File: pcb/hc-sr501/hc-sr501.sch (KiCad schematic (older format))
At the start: 35 parts, among them J1 Conector 3 pines, U1 BISS0001, U2 HT7133-1

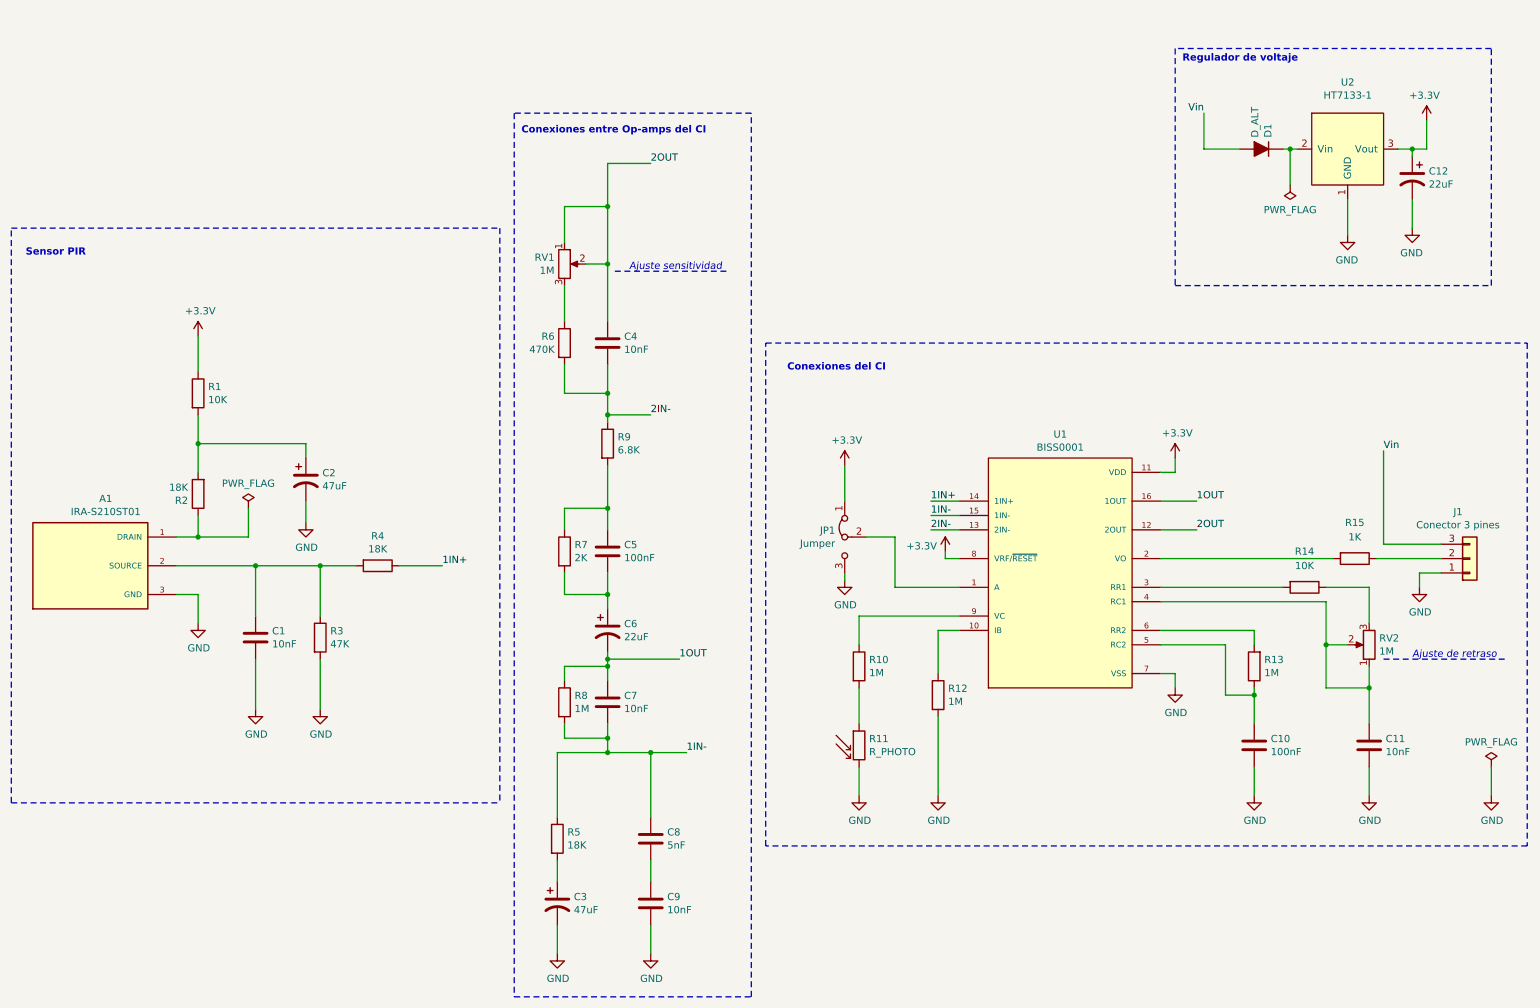
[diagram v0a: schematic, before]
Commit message: Cambios de PCB
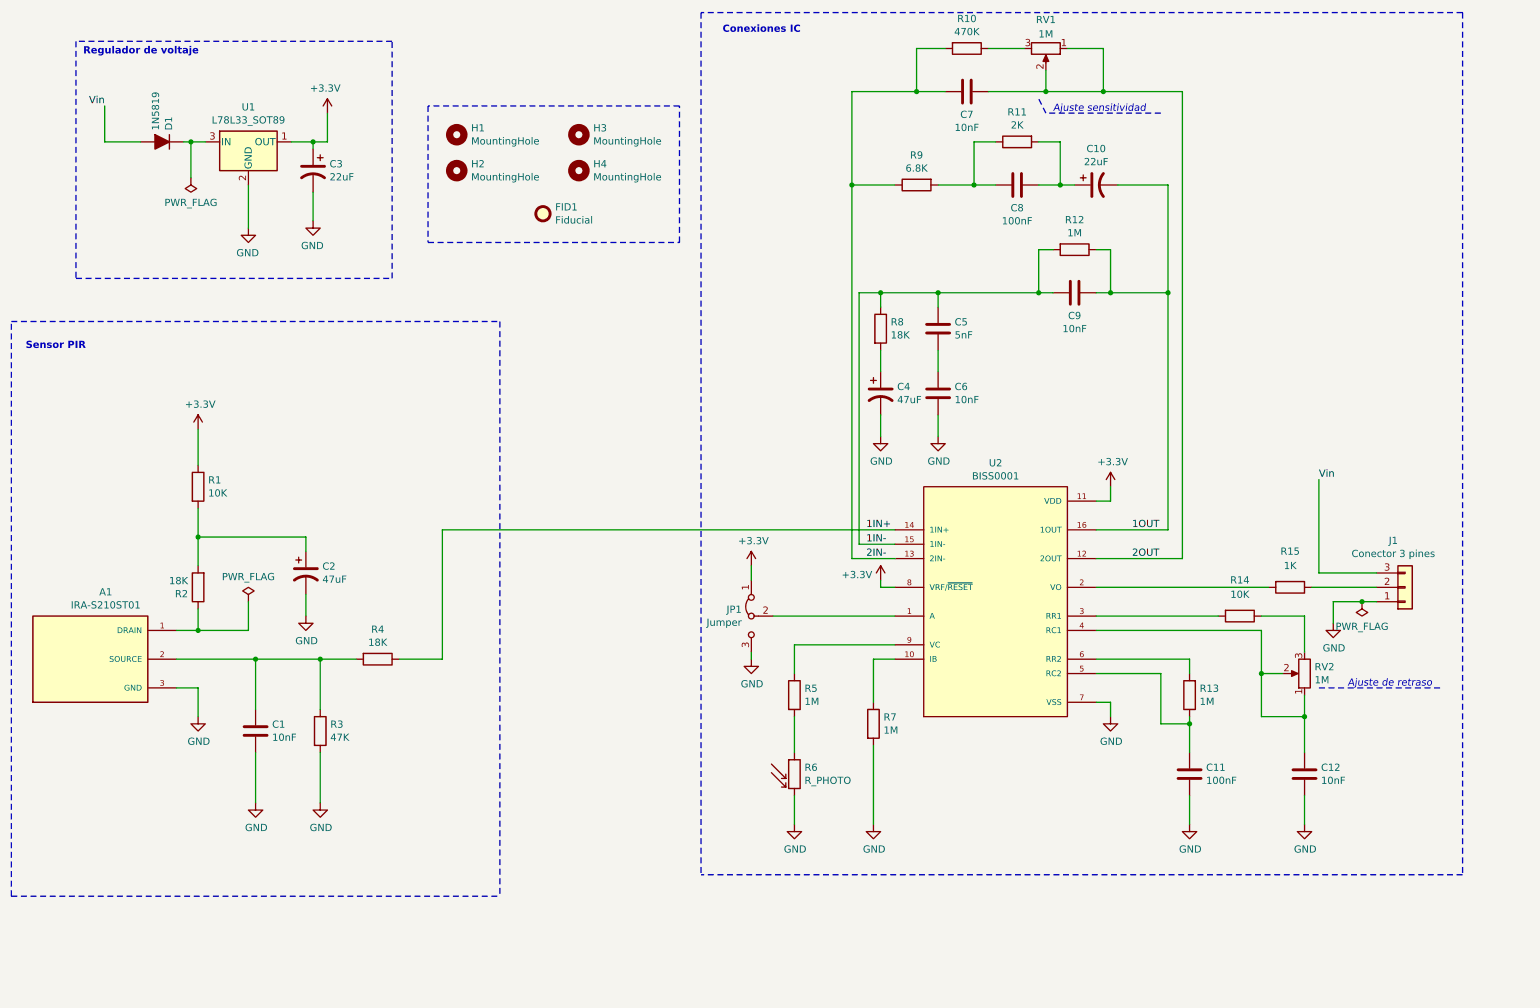
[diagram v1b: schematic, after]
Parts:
- removed U2: HT7133-1, Package_TO_SOT_SMD:SOT-89-3, symbol hc-sr501-rescue:HT7133-1-HT7133-1
- added FID1: Fiducial, Fiducial:Fiducial_0.5mm_Mask1mm, symbol Mechanical:Fiducial
- added H1, H2, H3, H4: MountingHole, myLib:MountingHole_1mm, symbol Mechanical:MountingHole
- added U1: L78L33_SOT89, Package_TO_SOT_SMD:SOT-89-3, symbol Regulator_Linear:L78L33_SOT89
- A1: Digi-Key Part Number (none) -> 490-11915-ND
- C1: footprint Capacitor_SMD:C_0402_1005Metric -> Capacitor_SMD:C_0805_2012Metric_Pad1.18x1.45mm_HandSolder
- C11: renamed from C10; footprint Capacitor_SMD:C_0402_1005Metric -> Capacitor_SMD:C_0805_2012Metric_Pad1.18x1.45mm_HandSolder
- C12: renamed from C11; footprint Capacitor_SMD:C_0402_1005Metric -> Capacitor_SMD:C_0805_2012Metric_Pad1.18x1.45mm_HandSolder
- C5: renamed from C8; footprint Capacitor_SMD:C_0402_1005Metric -> Capacitor_SMD:C_0805_2012Metric_Pad1.18x1.45mm_HandSolder
- C6: renamed from C9; footprint Capacitor_SMD:C_0402_1005Metric -> Capacitor_SMD:C_0805_2012Metric_Pad1.18x1.45mm_HandSolder
- C7: renamed from C4; footprint Capacitor_SMD:C_0402_1005Metric -> Capacitor_SMD:C_0805_2012Metric_Pad1.18x1.45mm_HandSolder
- C8: renamed from C5; footprint Capacitor_SMD:C_0402_1005Metric -> Capacitor_SMD:C_0805_2012Metric_Pad1.18x1.45mm_HandSolder
- C9: renamed from C7; footprint Capacitor_SMD:C_0402_1005Metric -> Capacitor_SMD:C_0805_2012Metric_Pad1.18x1.45mm_HandSolder
- D1: value D_ALT -> 1N5819
- JP1: footprint Jumper:SolderJumper-3_P1.3mm_Bridged2Bar12_Pad1.0x1.5mm_NumberLabels -> Jumper:SolderJumper-3_P1.3mm_Open_Pad1.0x1.5mm_NumberLabels
- R1, R13, R14, R15, R2, R3, R4, R9: footprint Resistor_SMD:R_0402_1005Metric -> Resistor_SMD:R_0805_2012Metric_Pad1.20x1.40mm_HandSolder
- R10: renamed from R6; footprint Resistor_SMD:R_0402_1005Metric -> Resistor_SMD:R_0805_2012Metric_Pad1.20x1.40mm_HandSolder
- R11: renamed from R7; footprint Resistor_SMD:R_0402_1005Metric -> Resistor_SMD:R_0805_2012Metric_Pad1.20x1.40mm_HandSolder
- R12: renamed from R8; footprint Resistor_SMD:R_0402_1005Metric -> Resistor_SMD:R_0805_2012Metric_Pad1.20x1.40mm_HandSolder
- R5: renamed from R10; footprint Resistor_SMD:R_0402_1005Metric -> Resistor_SMD:R_0805_2012Metric_Pad1.20x1.40mm_HandSolder
- R6: renamed from R11; footprint Resistor_SMD:R_0402_1005Metric -> Resistor_SMD:R_0805_2012Metric_Pad1.20x1.40mm_HandSolder
- R7: renamed from R12; footprint Resistor_SMD:R_0402_1005Metric -> Resistor_SMD:R_0805_2012Metric_Pad1.20x1.40mm_HandSolder
- R8: renamed from R5; footprint Resistor_SMD:R_0402_1005Metric -> Resistor_SMD:R_0805_2012Metric_Pad1.20x1.40mm_HandSolder
- RV1: Digi-Key Part Number (none) -> 3266W-101-ND
- RV2: Digi-Key Part Number  (none) -> 3266W-101-ND
- U2: renamed from U1; A1_MIN 0.1 -> (none); A_MAX 1.8 -> (none); A_MIN 1.8 -> (none); A_NOM 1.8 -> (none); B_MAX 0.45 -> (none); B_MIN 0.45 -> (none); B_NOM 0.45 -> (none); D2_MAX 0.0 -> (none); D_MAX 10.0 -> (none); D_MIN 10.0 -> (none); D_NOM 10.0 -> (none); E1_MAX 3.9 -> (none); E1_MIN 3.9 -> (none); E1_NOM 3.9 -> (none); E2_MAX 0.0 -> (none); ENOM 1.27 -> (none); E_MAX 6.0 -> (none); E_MIN 6.0 -> (none); E_NOM 6.0 -> (none); L_MAX 0.5 -> (none); L_MIN 0.5 -> (none); L_NOM 0.5 -> (none); Mouser N (none) -> 485-189; PIN_COUNT 16.0 -> (none)
- renumbered C6 to C10, C12 to C3, C3 to C4
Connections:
- net +3V3: now also U1.1 (OUT)
- net GND: now also U1.2 (GND)
- net at D1.1 (K): now also U1.3 (IN)
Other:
- note added: "Conexiones IC"
- note removed: "Conexiones del CI"
- note removed: "Conexiones entre Op-amps del CI"
- moved on the sheet: A1, C1, C10, C11, C12, C2, C3, C4, C5, C6, C7, C8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

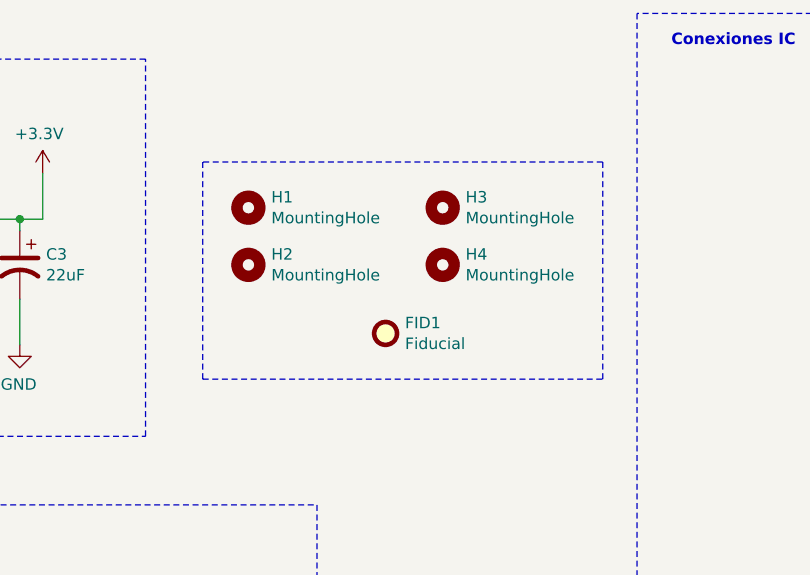
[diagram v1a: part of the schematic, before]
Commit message: PCB completo sin montaje
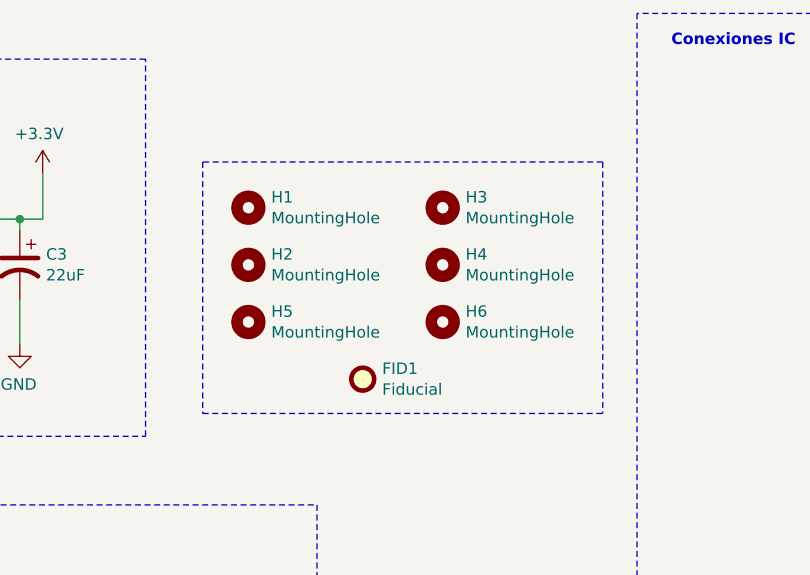
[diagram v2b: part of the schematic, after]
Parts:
- added H5, H6: MountingHole, MountingHole:MountingHole_2.1mm, symbol Mechanical:MountingHole
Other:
- moved on the sheet: FID1
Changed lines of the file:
@@
 L Mechanical:Fiducial FID1
 U 1 1 60AC52D1
-P 4300 1900
-F 0 "FID1" H 4385 1946 50  0000 L CNN
-F 1 "Fiducial" H 4385 1855 50  0000 L CNN
-F 2 "Fiducial:Fiducial_0.5mm_Mask1mm" H 4300 1900 50  0001 C CNN
-F 3 "~" H 4300 1900 50  0001 C CNN
-	1    4300 1900
+P 4200 2100
+F 0 "FID1" H 4285 2146 50  0000 L CNN
+F 1 "Fiducial" H 4285 2055 50  0000 L CNN
+F 2 "Fiducial:Fiducial_0.5mm_Mask1mm" H 4200 2100 50  0001 C CNN
+F 3 "~" H 4200 2100 50  0001 C CNN
+	1    4200 2100
 	1    0    0    -1
 $EndComp
 Wire Notes Line
-	3500 1150 3500 2100
-Wire Notes Line
-	3500 2100 5250 2100
-Wire Notes Line
-	5250 2100 5250 1150
+	3500 2250 5250 2250
 Wire Notes Line
 	5250 1150 3500 1150
@@
 Wire Wire Line
 	2250 1700 2250 2000
+$Comp
+L Mechanical:MountingHole H5
+U 1 1 609788D6
+P 3700 1850
+F 0 "H5" H 3800 1896 50  0000 L CNN
+F 1 "MountingHole" H 3800 1805 50  0000 L CNN
+F 2 "MountingHole:MountingHole_2.1mm" H 3700 1850 50  0001 C CNN
+F 3 "~" H 3700 1850 50  0001 C CNN
+	1    3700 1850
+	1    0    0    -1
+$EndComp
+$Comp
+L Mechanical:MountingHole H6
+U 1 1 609797D8
+P 4550 1850
+F 0 "H6" H 4650 1896 50  0000 L CNN
+F 1 "MountingHole" H 4650 1805 50  0000 L CNN
+F 2 "MountingHole:MountingHole_2.1mm" H 4550 1850 50  0001 C CNN
+F 3 "~" H 4550 1850 50  0001 C CNN
+	1    4550 1850
+	1    0    0    -1
+$EndComp
+Wire Notes Line
+	3500 1150 3500 2250
+Wire Notes Line
+	5250 1150 5250 2250
 $EndSCHEMATC
